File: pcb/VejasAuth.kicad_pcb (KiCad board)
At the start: 2 copper layers, 16.9 x 45.5 mm, 38 parts, among them J1 USB_A, J3 UP20-C-F-G-FL-P12-TR, SW1 SW_SPST, SW2 SW_SPST, U2 W25Q128JVS, U3 XC6206P332MR-G, U4 RP2350A-QFN60, Y1 ABM8-272-T3

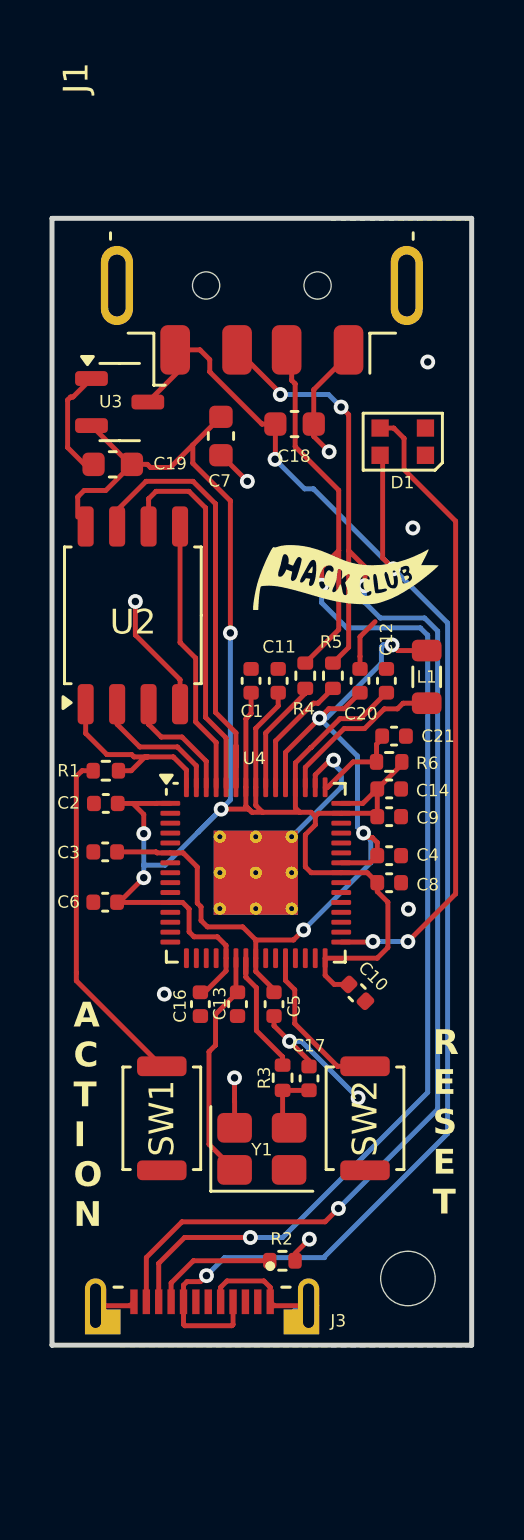
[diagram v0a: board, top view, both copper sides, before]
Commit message: big update
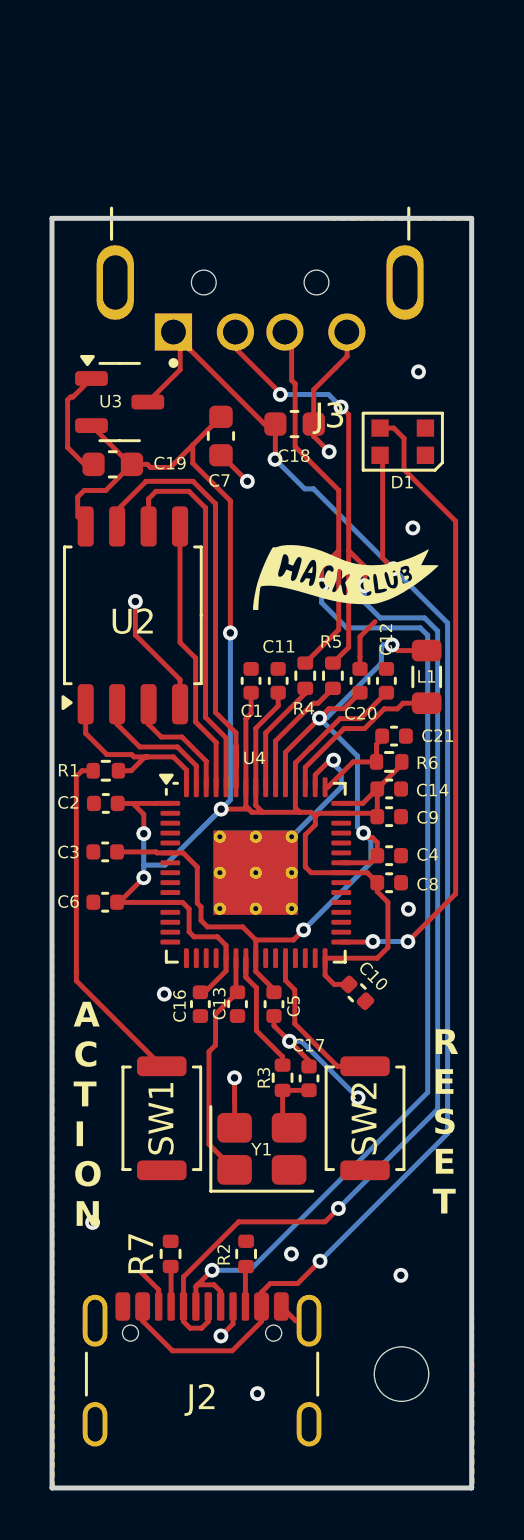
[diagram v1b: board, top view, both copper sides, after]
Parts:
- removed J1: USB_A, Connector_USB:USB_A_Molex_48037-2200_Horizontal
- added J2: USB_C_Receptacle_USB2.0_16P, Connector_USB:USB_C_Receptacle_GCT_USB4105-xx-A_16P_TopMnt_Horizontal, F.Cu at (161.3, 127.0)
- added R7: 5.1k, Resistor_SMD:R_0402_1005Metric, F.Cu at (160.0, 121.2)
- J3: value UP20-C-F-G-FL-P12-TR -> UP2-AH-4-TH; footprint footprint:SAMESKY_UP20-C-F-G-FL-P12-TR -> usb a tht:CUI_UP2-AH-4-TH
- moved J3 42.8 mm to (163.6, 82.0), turned to 180 degrees
- moved REF** 3.87 mm to (169.3, 126.1)
- moved R2 1.49 mm to (163.1, 121.2), turned to 90 degrees
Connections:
- R2 pad 1: Net-(J3-CC1) -> Net-(J2-CC2)
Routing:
- net Net-(J3-CC1): track 5.28 -> 0.00 mm
- net GND: track 42.5 -> 38.9 mm, vias 12 -> 16
- net Net-(J2-CC2): track 0.00 -> 1.62 mm
- net Net-(J2-CC1): track 0.00 -> 1.62 mm
- net VBUS: track 62.2 -> 63.3 mm
- net /D-: track 57.2 -> 57.7 mm
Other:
- board size 16.9 x 45.5 mm -> 16.9 x 51.3 mm
